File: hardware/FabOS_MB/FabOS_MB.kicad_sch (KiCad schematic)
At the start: 4 parts

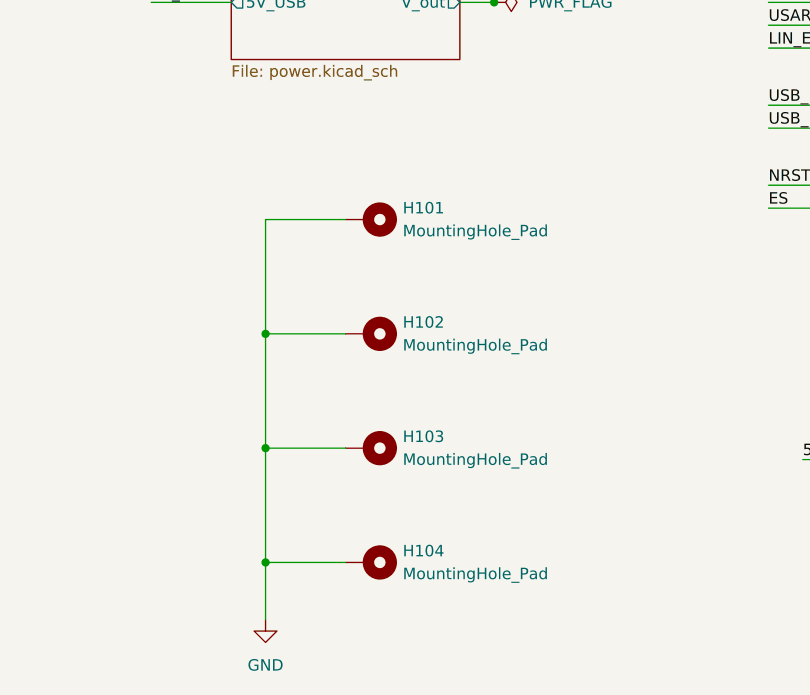
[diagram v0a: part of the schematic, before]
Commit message: create pcb
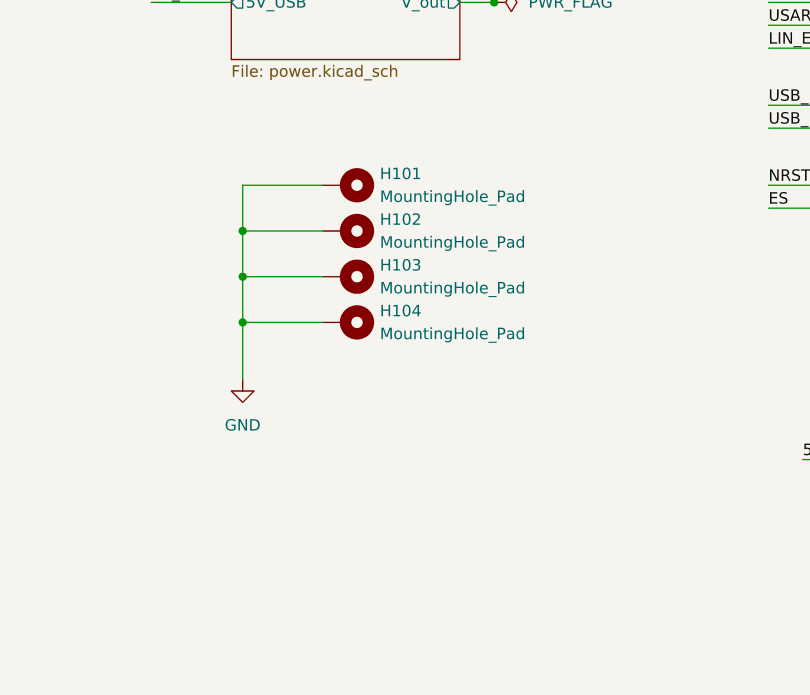
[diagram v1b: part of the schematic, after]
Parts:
- H101, H102, H103, H104: footprint MountingHole:MountingHole_3.2mm_M3_DIN965_Pad -> MountingHole:MountingHole_3.2mm_M3_Pad_Via
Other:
- moved on the sheet: H101, H102, H103, H104
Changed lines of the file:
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@@
 	)
 	(junction
-		(at 41.91 93.98)
+		(at 39.37 67.31)
 		(diameter 0)
 		(color 0 0 0 0)
 	)
 	(junction
-		(at 41.91 68.58)
+		(at 39.37 57.15)
 		(diameter 0)
 		(color 0 0 0 0)
 	)
 	(junction
-		(at 41.91 81.28)
+		(at 39.37 62.23)
 		(diameter 0)
 		(color 0 0 0 0)
@@
 	(wire
 		(pts
-			(xy 50.8 55.88) (xy 41.91 55.88)
+			(xy 48.26 52.07) (xy 39.37 52.07)
 		)
 		(stroke
@@
 	(wire
 		(pts
-			(xy 41.91 93.98) (xy 50.8 93.98)
-		)
-		(stroke
-			(width 0)
-			(type default)
-		)
-	)
-	(wire
-		(pts
-			(xy 41.91 68.58) (xy 41.91 81.28)
-		)
-		(stroke
-			(width 0)
-			(type default)
-		)
-	)
-	(wire
-		(pts
-			(xy 41.91 68.58) (xy 50.8 68.58)
+			(xy 39.37 67.31) (xy 48.26 67.31)
+		)
+		(stroke
+			(width 0)
+			(type default)
+		)
+	)
+	(wire
+		(pts
+			(xy 39.37 57.15) (xy 39.37 62.23)
+		)
+		(stroke
+			(width 0)
+			(type default)
+		)
+	)
+	(wire
+		(pts
+			(xy 39.37 57.15) (xy 48.26 57.15)
 		)
 		(stroke
@@
 	(wire
 		(pts
-			(xy 41.91 93.98) (xy 41.91 100.33)
+			(xy 39.37 67.31) (xy 39.37 73.66)
 		)
 		(stroke
@@
 	(wire
 		(pts
-			(xy 41.91 81.28) (xy 50.8 81.28)
-		)
-		(stroke
-			(width 0)
-			(type default)
-		)
-	)
-	(wire
-		(pts
-			(xy 41.91 55.88) (xy 41.91 68.58)
+			(xy 39.37 62.23) (xy 48.26 62.23)
+		)
+		(stroke
+			(width 0)
+			(type default)
+		)
+	)
+	(wire
+		(pts
+			(xy 39.37 52.07) (xy 39.37 57.15)
 		)
 		(stroke
@@
 	(wire
 		(pts
-			(xy 41.91 81.28) (xy 41.91 93.98)
+			(xy 39.37 62.23) (xy 39.37 67.31)
 		)
 		(stroke
@@
 	(symbol
 		(lib_id "Mechanical:MountingHole_Pad")
-		(at 53.34 55.88 270)
+		(at 50.8 52.07 270)
 		(unit 1)
 		(exclude_from_sim yes)
@@
 		(fields_autoplaced yes)
 		(property "Reference" "H101"
-			(at 57.15 54.6099 90)
+			(at 54.61 50.7999 90)
 			(effects
 				(font
@@
 		)
 		(property "Value" "MountingHole_Pad"
-			(at 57.15 57.1499 90)
+			(at 54.61 53.3399 90)
 			(effects
 				(font
@@
 			)
 		)
-		(property "Footprint" "MountingHole:MountingHole_3.2mm_M3_DIN965_Pad"
-			(at 53.34 55.88 0)
+		(property "Footprint" "MountingHole:MountingHole_3.2mm_M3_Pad_Via"
+			(at 50.8 52.07 0)
 			(effects
 				(font
@@
 		)
 		(property "Datasheet" "~"
-			(at 53.34 55.88 0)
+			(at 50.8 52.07 0)
 			(effects
 				(font
@@
 		)
 		(property "Description" "Mounting Hole with connection"
-			(at 53.34 55.88 0)
+			(at 50.8 52.07 0)
 			(effects
 				(font
@@
 	(symbol
 		(lib_id "Mechanical:MountingHole_Pad")
-		(at 53.34 81.28 270)
+		(at 50.8 62.23 270)
 		(unit 1)
 		(exclude_from_sim yes)
@@
 		(fields_autoplaced yes)
 		(property "Reference" "H103"
-			(at 57.15 80.0099 90)
+			(at 54.61 60.9599 90)
 			(effects
 				(font
@@
 		)
 		(property "Value" "MountingHole_Pad"
-			(at 57.15 82.5499 90)
+			(at 54.61 63.4999 90)
 			(effects
 				(font
@@
 			)
 		)
-		(property "Footprint" "MountingHole:MountingHole_3.2mm_M3_DIN965_Pad"
-			(at 53.34 81.28 0)
+		(property "Footprint" "MountingHole:MountingHole_3.2mm_M3_Pad_Via"
+			(at 50.8 62.23 0)
 			(effects
 				(font
@@
 		)
 		(property "Datasheet" "~"
-			(at 53.34 81.28 0)
+			(at 50.8 62.23 0)
 			(effects
 				(font
@@
 		)
 		(property "Description" "Mounting Hole with connection"
-			(at 53.34 81.28 0)
+			(at 50.8 62.23 0)
 			(effects
 				(font
@@
 	(symbol
 		(lib_id "power:GND")
-		(at 41.91 100.33 0)
+		(at 39.37 73.66 0)
 		(unit 1)
 		(exclude_from_sim no)
@@
 		(fields_autoplaced yes)
 		(property "Reference" "#PWR0101"
-			(at 41.91 106.68 0)
+			(at 39.37 80.01 0)
 			(effects
 				(font
@@
 		)
 		(property "Value" "GND"
-			(at 41.91 105.41 0)
+			(at 39.37 78.74 0)
 			(effects
 				(font
@@
 		)
 		(property "Footprint" ""
-			(at 41.91 100.33 0)
+			(at 39.37 73.66 0)
 			(effects
 				(font
@@
 		)
 		(property "Datasheet" ""
-			(at 41.91 100.33 0)
+			(at 39.37 73.66 0)
 			(effects
 				(font
@@
 		)
 		(property "Description" "Power symbol creates a global label with name \"GND\" , ground"
-			(at 41.91 100.33 0)
+			(at 39.37 73.66 0)
 			(effects
 				(font
@@
 	(symbol
 		(lib_id "Mechanical:MountingHole_Pad")
-		(at 53.34 68.58 270)
+		(at 50.8 57.15 270)
 		(unit 1)
 		(exclude_from_sim yes)
@@
 		(fields_autoplaced yes)
 		(property "Reference" "H102"
-			(at 57.15 67.3099 90)
+			(at 54.61 55.8799 90)
 			(effects
 				(font
@@
 		)
 		(property "Value" "MountingHole_Pad"
-			(at 57.15 69.8499 90)
+			(at 54.61 58.4199 90)
 			(effects
 				(font
@@
 			)
 		)
-		(property "Footprint" "MountingHole:MountingHole_3.2mm_M3_DIN965_Pad"
-			(at 53.34 68.58 0)
+		(property "Footprint" "MountingHole:MountingHole_3.2mm_M3_Pad_Via"
+			(at 50.8 57.15 0)
 			(effects
 				(font
@@
 		)
 		(property "Datasheet" "~"
-			(at 53.34 68.58 0)
+			(at 50.8 57.15 0)
 			(effects
 				(font
@@
 		)
 		(property "Description" "Mounting Hole with connection"
-			(at 53.34 68.58 0)
+			(at 50.8 57.15 0)
 			(effects
 				(font
@@
 	(symbol
 		(lib_id "Mechanical:MountingHole_Pad")
-		(at 53.34 93.98 270)
+		(at 50.8 67.31 270)
 		(unit 1)
 		(exclude_from_sim yes)
@@
 		(fields_autoplaced yes)
 		(property "Reference" "H104"
-			(at 57.15 92.7099 90)
+			(at 54.61 66.0399 90)
 			(effects
 				(font
@@
 		)
 		(property "Value" "MountingHole_Pad"
-			(at 57.15 95.2499 90)
+			(at 54.61 68.5799 90)
 			(effects
 				(font
@@
 			)
 		)
-		(property "Footprint" "MountingHole:MountingHole_3.2mm_M3_DIN965_Pad"
-			(at 53.34 93.98 0)
+		(property "Footprint" "MountingHole:MountingHole_3.2mm_M3_Pad_Via"
+			(at 50.8 67.31 0)
 			(effects
 				(font
@@
 		)
 		(property "Datasheet" "~"
-			(at 53.34 93.98 0)
+			(at 50.8 67.31 0)
 			(effects
 				(font
@@
 		)
 		(property "Description" "Mounting Hole with connection"
-			(at 53.34 93.98 0)
-			(effects
-				(font
+			(at 50.8 67.31 0)
+			(effects
+				(font
